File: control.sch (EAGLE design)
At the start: 39 parts, among them IC1 OPA336P, IC2 XMEGA16A4A, IC3 LM317MBSTT3, Q1 BSS92, Q2 BSS101

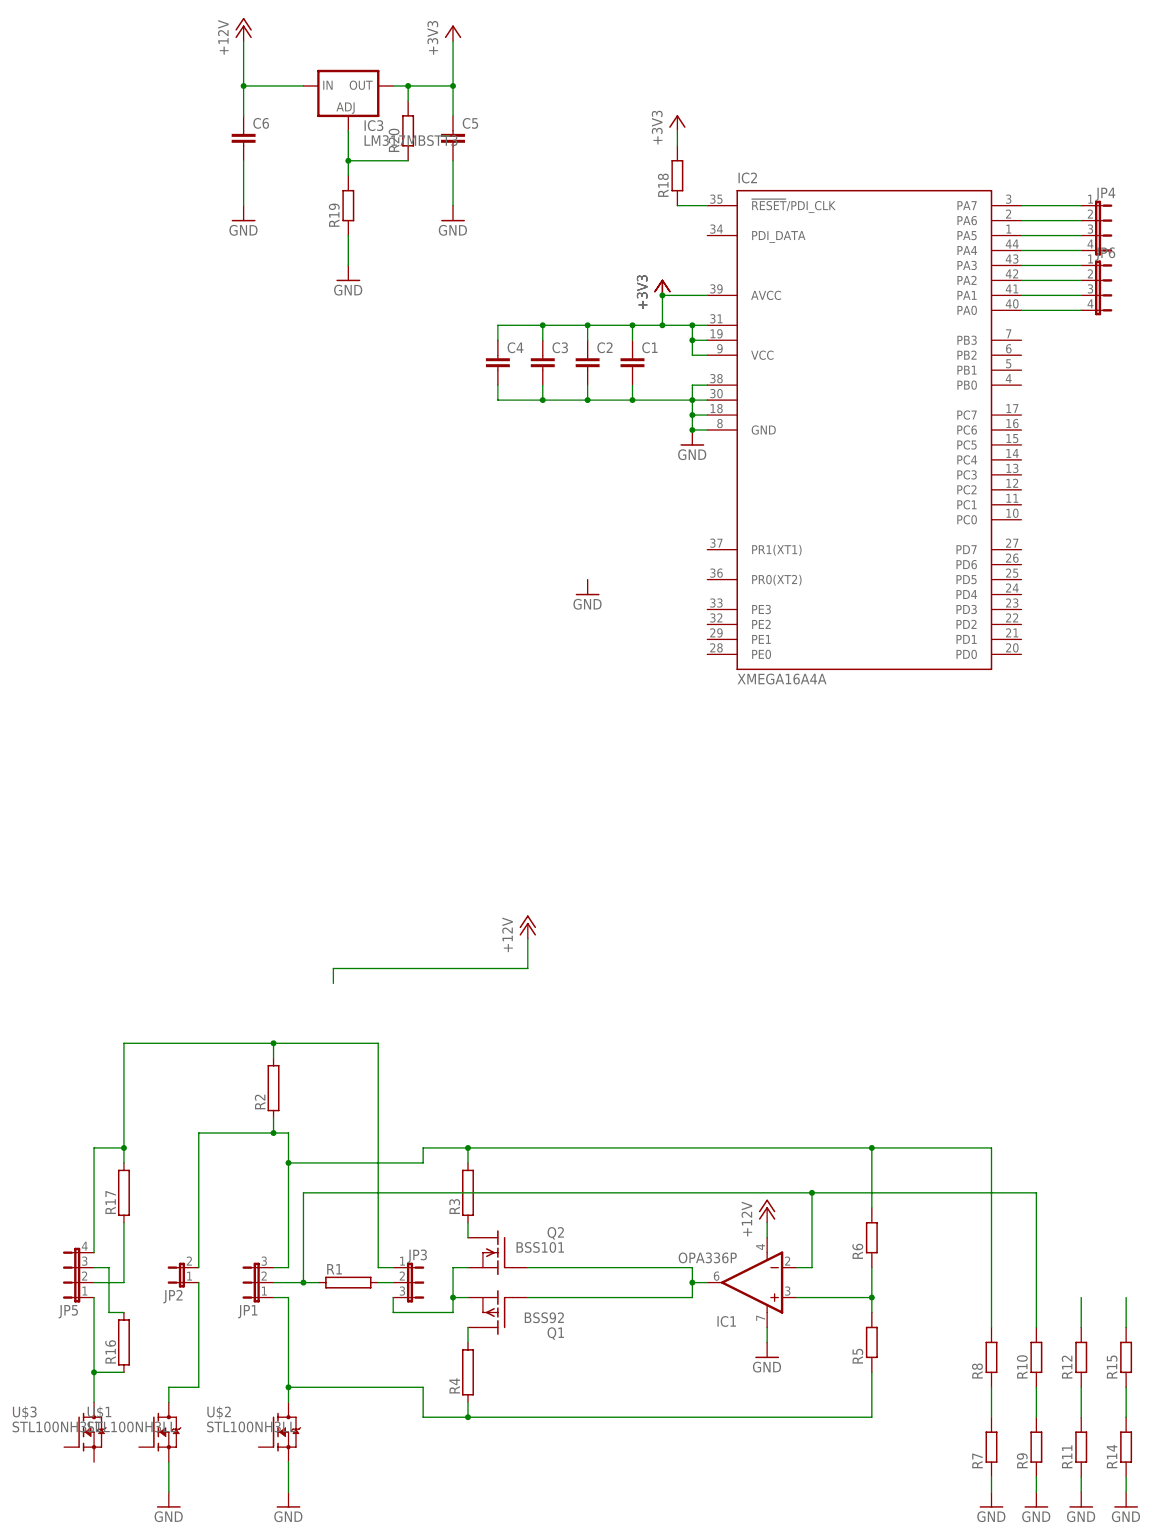
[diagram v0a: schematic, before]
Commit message: +spannungsregler
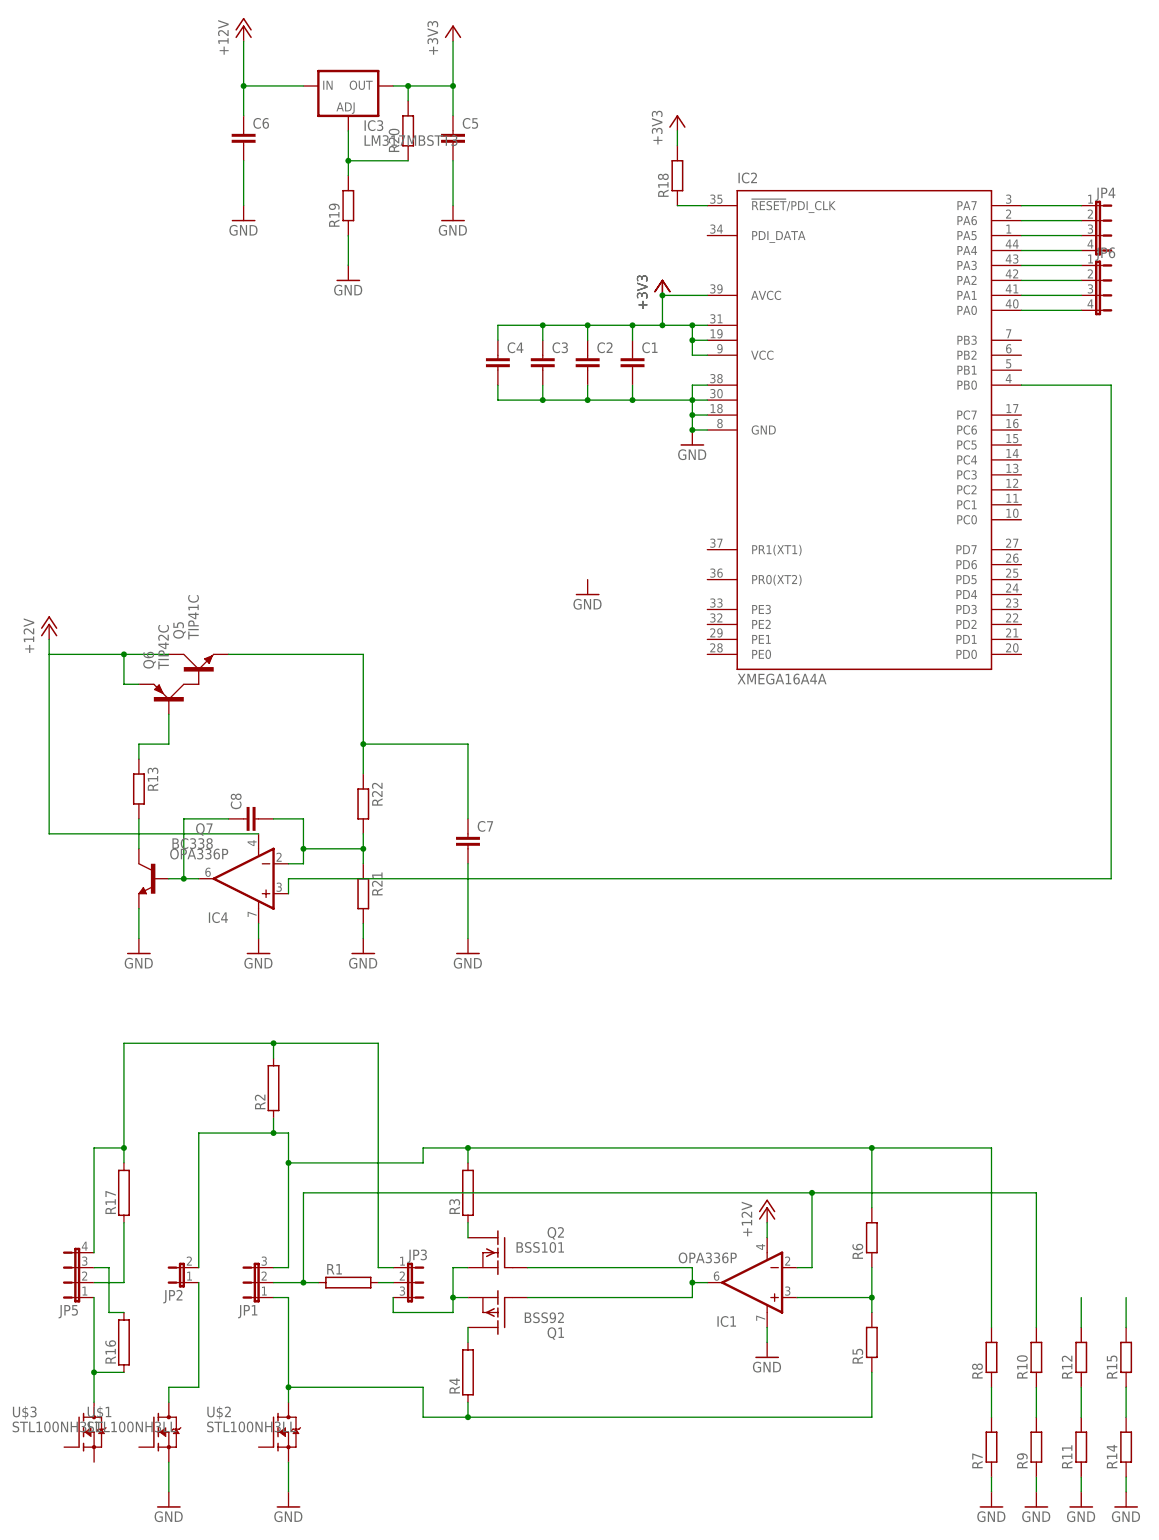
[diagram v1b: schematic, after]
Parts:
- added C7, C8: (no value), resistor:C-EUC0805K
- added IC4: OPA336P, burr-brown:OPA336P
- added Q5: TIP41C, transistor-power:TIP41C
- added Q6: TIP42C, transistor-power:TIP42C
- added Q7: BC338, transistor-npn:BC338
- added R13, R21, R22: (no value), resistor:R-EU_M0805
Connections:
- new net N$12: C7.1, Q5.E, R22.1
- new net N$13: Q7.C, R13.2
- new net N$26: Q6.B, R13.1
- new net N$28: C8.1, IC4.OUT, Q7.B
- new net N$30: C8.2, IC4.-IN, R21.1, R22.2
- new net N$31: IC2.PB0, IC4.+IN
- new net N$32: Q5.B, Q6.C
- net +12V: now also IC4.V-, Q5.C, Q6.E
- net GND: now also C7.2, IC4.V+, Q7.E, R21.2
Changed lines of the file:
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@@
 <part name="JP4" library="jumper" deviceset="JP4E" device=""/>
 <part name="JP6" library="jumper" deviceset="JP4E" device=""/>
+<part name="R13" library="resistor" deviceset="R-EU_" device="M0805"/>
+<part name="IC4" library="burr-brown" deviceset="OPA336" device="P"/>
+<part name="R21" library="resistor" deviceset="R-EU_" device="M0805"/>
+<part name="R22" library="resistor" deviceset="R-EU_" device="M0805"/>
+<part name="C7" library="resistor" deviceset="C-EU" device="C0805K"/>
+<part name="C8" library="resistor" deviceset="C-EU" device="C0805K"/>
+<part name="GND13" library="supply1" deviceset="GND" device=""/>
+<part name="GND14" library="supply1" deviceset="GND" device=""/>
+<part name="GND15" library="supply1" deviceset="GND" device=""/>
+<part name="GND16" library="supply1" deviceset="GND" device=""/>
+<part name="Q5" library="transistor-power" deviceset="TIP41C" device=""/>
+<part name="Q6" library="transistor-power" deviceset="TIP42C" device=""/>
+<part name="Q7" library="transistor-npn" deviceset="BC338*" device=""/>
 </parts>
 <sheets>
@@
 <instance part="GND2" gate="1" x="33.02" y="15.24"/>
 <instance part="GND3" gate="1" x="114.3" y="40.64"/>
-<instance part="P+1" gate="1" x="73.66" y="114.3"/>
+<instance part="P+1" gate="1" x="-7.62" y="165.1"/>
 <instance part="P+2" gate="1" x="114.3" y="66.04"/>
 <instance part="R7" gate="G$1" x="152.4" y="25.4" rot="R90"/>
@@
 <instance part="JP4" gate="G$1" x="170.18" y="233.68" rot="R270"/>
 <instance part="JP6" gate="G$1" x="170.18" y="223.52" rot="R270"/>
+<instance part="R13" gate="G$1" x="7.62" y="137.16" rot="R270"/>
+<instance part="IC4" gate="G$1" x="25.4" y="121.92" rot="R180"/>
+<instance part="R21" gate="G$1" x="45.72" y="119.38" rot="R270"/>
+<instance part="R22" gate="G$1" x="45.72" y="134.62" rot="R270"/>
+<instance part="C7" gate="G$1" x="63.5" y="129.54"/>
+<instance part="C8" gate="G$1" x="25.4" y="132.08" rot="R90"/>
+<instance part="GND13" gate="1" x="45.72" y="109.22"/>
+<instance part="GND14" gate="1" x="27.94" y="109.22"/>
+<instance part="GND15" gate="1" x="7.62" y="109.22"/>
+<instance part="GND16" gate="1" x="63.5" y="109.22"/>
+<instance part="Q5" gate="1" x="17.78" y="157.48" rot="R90"/>
+<instance part="Q6" gate="1" x="12.7" y="152.4" rot="R90"/>
+<instance part="Q7" gate="G$1" x="10.16" y="121.92" rot="MR0"/>
 </instances>
 <busses>
@@
 <wire x1="25.4" y1="236.22" x2="25.4" y2="243.84" width="0.1524" layer="91"/>
 </segment>
+<segment>
+<pinref part="IC4" gate="G$1" pin="V+"/>
+<pinref part="GND14" gate="1" pin="GND"/>
+<wire x1="27.94" y1="114.3" x2="27.94" y2="111.76" width="0.1524" layer="91"/>
+</segment>
+<segment>
+<pinref part="R21" gate="G$1" pin="2"/>
+<pinref part="GND13" gate="1" pin="GND"/>
+<wire x1="45.72" y1="114.3" x2="45.72" y2="111.76" width="0.1524" layer="91"/>
+</segment>
+<segment>
+<pinref part="GND16" gate="1" pin="GND"/>
+<pinref part="C7" gate="G$1" pin="2"/>
+<wire x1="63.5" y1="111.76" x2="63.5" y2="124.46" width="0.1524" layer="91"/>
+</segment>
+<segment>
+<pinref part="Q7" gate="G$1" pin="E"/>
+<pinref part="GND15" gate="1" pin="GND"/>
+<wire x1="7.62" y1="111.76" x2="7.62" y2="116.84" width="0.1524" layer="91"/>
+</segment>
 </net>
 <net name="+12V" class="0">
@@
 <pinref part="P+2" gate="1" pin="+12V"/>
 <wire x1="114.3" y1="60.96" x2="114.3" y2="63.5" width="0.1524" layer="91"/>
-</segment>
-<segment>
-<pinref part="P+1" gate="1" pin="+12V"/>
-<wire x1="73.66" y1="111.76" x2="73.66" y2="106.68" width="0.1524" layer="91"/>
-<wire x1="73.66" y1="106.68" x2="40.64" y2="106.68" width="0.1524" layer="91"/>
-<wire x1="40.64" y1="106.68" x2="40.64" y2="104.14" width="0.1524" layer="91"/>
 </segment>
 <segment>
@@
 <wire x1="25.4" y1="256.54" x2="25.4" y2="264.16" width="0.1524" layer="91"/>
 <junction x="25.4" y="256.54"/>
+</segment>
+<segment>
+<pinref part="P+1" gate="1" pin="+12V"/>
+<wire x1="-7.62" y1="160.02" x2="-7.62" y2="162.56" width="0.1524" layer="91"/>
+<wire x1="-7.62" y1="160.02" x2="-7.62" y2="129.54" width="0.1524" layer="91"/>
+<pinref part="IC4" gate="G$1" pin="V-"/>
+<wire x1="27.94" y1="129.54" x2="-7.62" y2="129.54" width="0.1524" layer="91"/>
+<pinref part="Q5" gate="1" pin="C"/>
+<wire x1="12.7" y1="160.02" x2="5.08" y2="160.02" width="0.1524" layer="91"/>
+<wire x1="5.08" y1="160.02" x2="5.08" y2="154.94" width="0.1524" layer="91"/>
+<pinref part="Q6" gate="1" pin="E"/>
+<wire x1="5.08" y1="154.94" x2="7.62" y2="154.94" width="0.1524" layer="91"/>
+<wire x1="5.08" y1="160.02" x2="-7.62" y2="160.02" width="0.1524" layer="91"/>
+<junction x="5.08" y="160.02"/>
 </segment>
 </net>
@@
 </segment>
 </net>
+<net name="N$12" class="0">
+<segment>
+<pinref part="C7" gate="G$1" pin="1"/>
+<wire x1="45.72" y1="144.78" x2="63.5" y2="144.78" width="0.1524" layer="91"/>
+<wire x1="63.5" y1="144.78" x2="63.5" y2="132.08" width="0.1524" layer="91"/>
+<pinref part="R22" gate="G$1" pin="1"/>
+<wire x1="45.72" y1="139.7" x2="45.72" y2="144.78" width="0.1524" layer="91"/>
+<pinref part="Q5" gate="1" pin="E"/>
+<wire x1="22.86" y1="160.02" x2="45.72" y2="160.02" width="0.1524" layer="91"/>
+<wire x1="45.72" y1="160.02" x2="45.72" y2="144.78" width="0.1524" layer="91"/>
+<junction x="45.72" y="144.78"/>
+</segment>
+</net>
+<net name="N$28" class="0">
+<segment>
+<pinref part="IC4" gate="G$1" pin="OUT"/>
+<wire x1="17.78" y1="121.92" x2="15.24" y2="121.92" width="0.1524" layer="91"/>
+<wire x1="15.24" y1="121.92" x2="12.7" y2="121.92" width="0.1524" layer="91"/>
+<wire x1="15.24" y1="121.92" x2="15.24" y2="132.08" width="0.1524" layer="91"/>
+<junction x="15.24" y="121.92"/>
+<pinref part="C8" gate="G$1" pin="1"/>
+<wire x1="15.24" y1="132.08" x2="22.86" y2="132.08" width="0.1524" layer="91"/>
+<pinref part="Q7" gate="G$1" pin="B"/>
+</segment>
+</net>
+<net name="N$30" class="0">
+<segment>
+<pinref part="IC4" gate="G$1" pin="-IN"/>
+<wire x1="33.02" y1="124.46" x2="35.56" y2="124.46" width="0.1524" layer="91"/>
+<wire x1="35.56" y1="124.46" x2="35.56" y2="127" width="0.1524" layer="91"/>
+<pinref part="C8" gate="G$1" pin="2"/>
+<wire x1="35.56" y1="127" x2="35.56" y2="132.08" width="0.1524" layer="91"/>
+<wire x1="35.56" y1="132.08" x2="30.48" y2="132.08" width="0.1524" layer="91"/>
+<pinref part="R22" gate="G$1" pin="2"/>
+<pinref part="R21" gate="G$1" pin="1"/>
+<wire x1="45.72" y1="129.54" x2="45.72" y2="127" width="0.1524" layer="91"/>
+<wire x1="45.72" y1="127" x2="45.72" y2="124.46" width="0.1524" layer="91"/>
+<wire x1="35.56" y1="127" x2="45.72" y2="127" width="0.1524" layer="91"/>
+<junction x="35.56" y="127"/>
+<junction x="45.72" y="127"/>
+</segment>
+</net>
+<net name="N$31" class="0">
+<segment>
+<pinref part="IC2" gate="G$1" pin="PB0"/>
+<wire x1="157.48" y1="205.74" x2="172.72" y2="205.74" width="0.1524" layer="91"/>
+<wire x1="172.72" y1="205.74" x2="172.72" y2="121.92" width="0.1524" layer="91"/>
+<pinref part="IC4" gate="G$1" pin="+IN"/>
+<wire x1="172.72" y1="121.92" x2="33.02" y2="121.92" width="0.1524" layer="91"/>
+<wire x1="33.02" y1="121.92" x2="33.02" y2="119.38" width="0.1524" layer="91"/>
+</segment>
+</net>
+<net name="N$32" class="0">
+<segment>
+<pinref part="Q5" gate="1" pin="B"/>
+<pinref part="Q6" gate="1" pin="C"/>
+</segment>
+</net>
+<net name="N$13" class="0">
+<segment>
+<pinref part="Q7" gate="G$1" pin="C"/>
+<pinref part="R13" gate="G$1" pin="2"/>
+<wire x1="7.62" y1="132.08" x2="7.62" y2="127" width="0.1524" layer="91"/>
+</segment>
+</net>
+<net name="N$26" class="0">
+<segment>
+<pinref part="R13" gate="G$1" pin="1"/>
+<wire x1="7.62" y1="142.24" x2="7.62" y2="144.78" width="0.1524" layer="91"/>
+<pinref part="Q6" gate="1" pin="B"/>
+<wire x1="7.62" y1="144.78" x2="12.7" y2="144.78" width="0.1524" layer="91"/>
+<wire x1="12.7" y1="144.78" x2="12.7" y2="149.86" width="0.1524" layer="91"/>
+</segment>
+</net>
